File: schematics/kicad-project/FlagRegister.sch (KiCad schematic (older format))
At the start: 36 parts

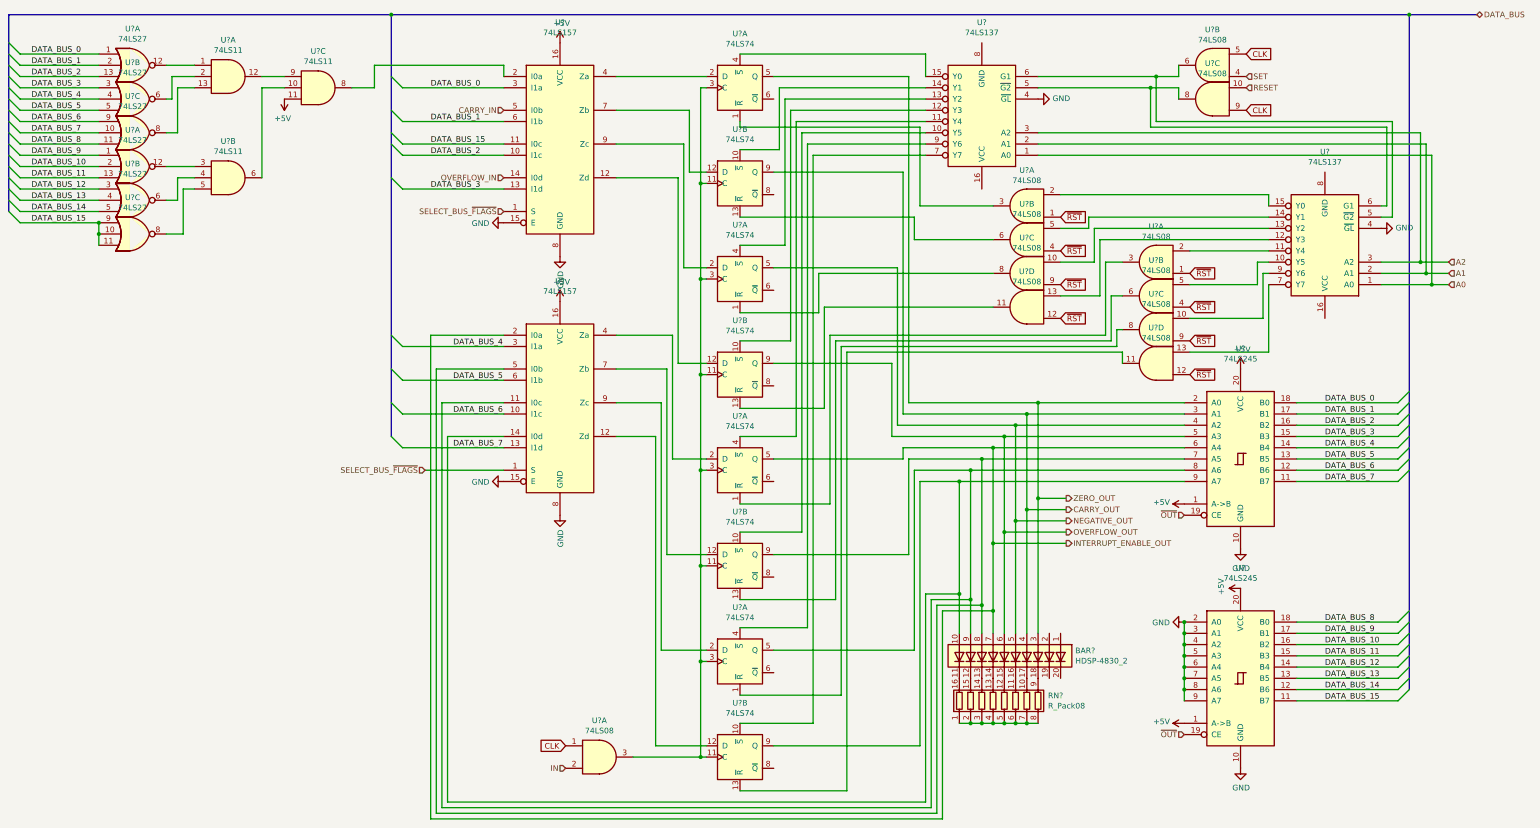
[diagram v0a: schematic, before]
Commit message: Update schematics
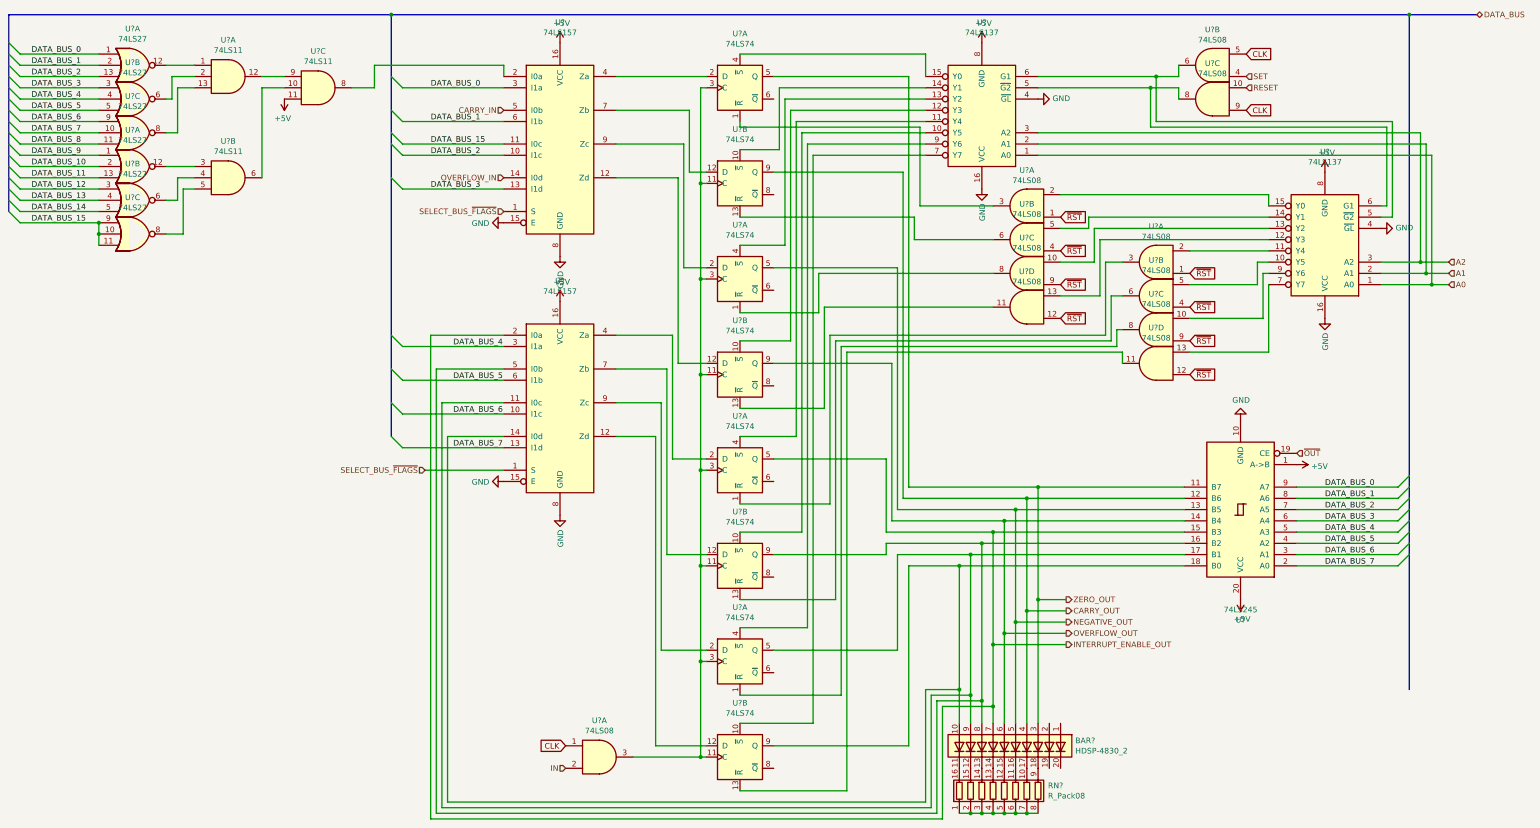
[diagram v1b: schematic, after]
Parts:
- removed U?: 74LS245, symbol 74xx:74LS245
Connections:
- net +5V: now also U?.8 (GND), U?.8 (GND)
- net CARRY_OUT: now also U?.12 (B6); no longer U?.3 (A1)
- net DATA_BUS_0: now also U?.9 (A7); no longer U?.18 (B0)
- net DATA_BUS_1: now also U?.8 (A6); no longer U?.17 (B1)
- net DATA_BUS_2: now also U?.7 (A5); no longer U?.16 (B2)
- net DATA_BUS_3: now also U?.6 (A4); no longer U?.15 (B3)
- net DATA_BUS_4: now also U?.5 (A3); no longer U?.14 (B4)
- net DATA_BUS_5: now also U?.4 (A2); no longer U?.13 (B5)
- net DATA_BUS_6: now also U?.3 (A1); no longer U?.12 (B6)
- net DATA_BUS_7: now also U?.2 (A0); no longer U?.11 (B7)
- net GND: now also U?.16 (VCC), U?.16 (VCC)
- net INTERRUPT_ENABLE_OUT: now also U?.15 (B3); no longer U?.6 (A4)
- net NEGATIVE_OUT: now also U?.13 (B5); no longer U?.4 (A2)
- net OVERFLOW_OUT: now also U?.14 (B4); no longer U?.5 (A3)
- net ZERO_OUT: now also U?.11 (B7); no longer U?.2 (A0)
- net at BAR?.9 (A), U?.11 (I0c), U?.5 (Q): now also U?.17 (B1); no longer U?.8 (A6)
- net at BAR?.10 (A), U?.14 (I0d), U?.9 (Q): now also U?.18 (B0); no longer U?.9 (A7)
- net at BAR?.8 (A), U?.5 (I0b), U?.9 (Q): now also U?.16 (B2); no longer U?.7 (A5)
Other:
- moved on the sheet: BAR?, RN?, U?
